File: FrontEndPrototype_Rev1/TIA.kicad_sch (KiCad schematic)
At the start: 10 parts, among them U14 LTC6252, U15 ADA4807-1

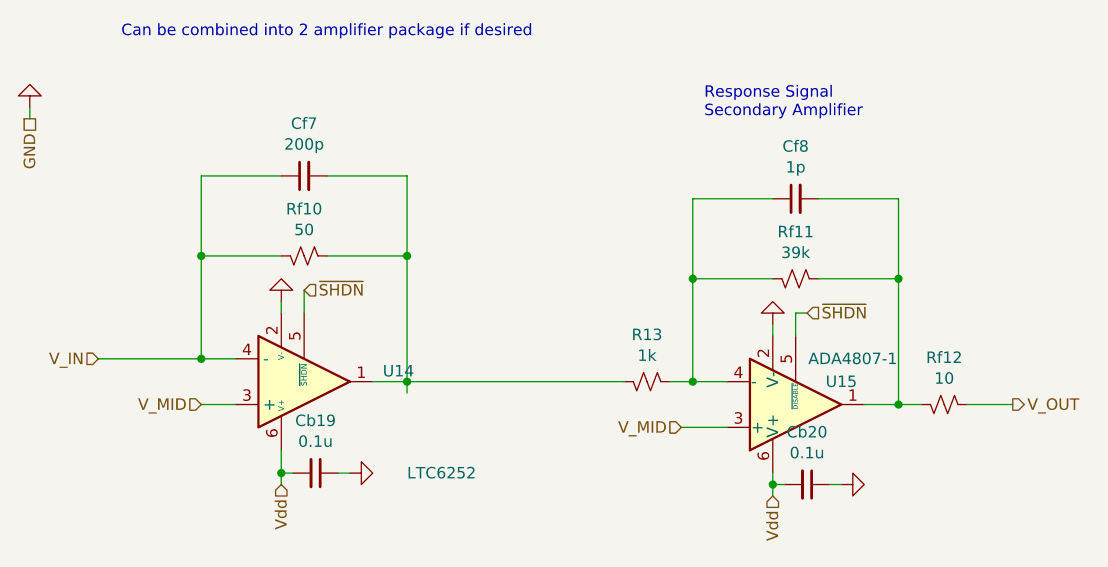
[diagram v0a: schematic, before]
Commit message: First Pass Schematic Fixes for Power Management Board
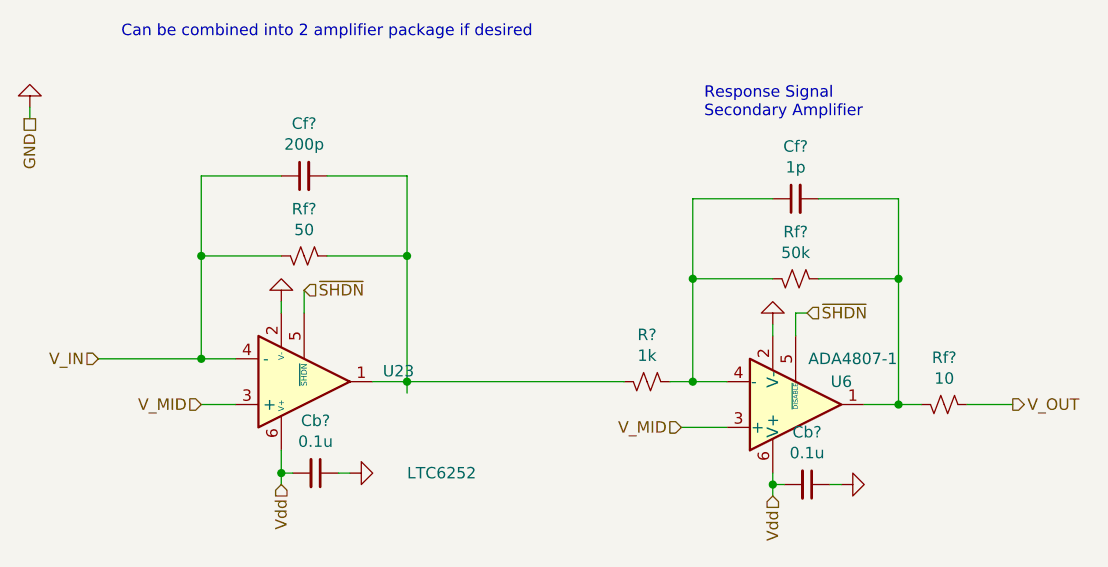
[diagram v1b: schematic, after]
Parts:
- Rf?: renamed from Rf11; value 39k -> 50k
- renumbered Cb20 to Cb?, Cb19 to Cb?, Cf7 to Cf?, Cf8 to Cf?, R13 to R?, Rf12 to Rf?, Rf10 to Rf?, U14 to U23, U15 to U6
